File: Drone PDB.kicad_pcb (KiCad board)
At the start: 2 copper layers, 8 parts, among them CN1 XT60PW-M, CN2 XT60PW-M, CN3 XT60PW-M, CN4 XT60PW-M, CN5 XT60PW-M, CN6 XT60PW-M, CN7 XT60PW-M, CN8 XT60PW-M

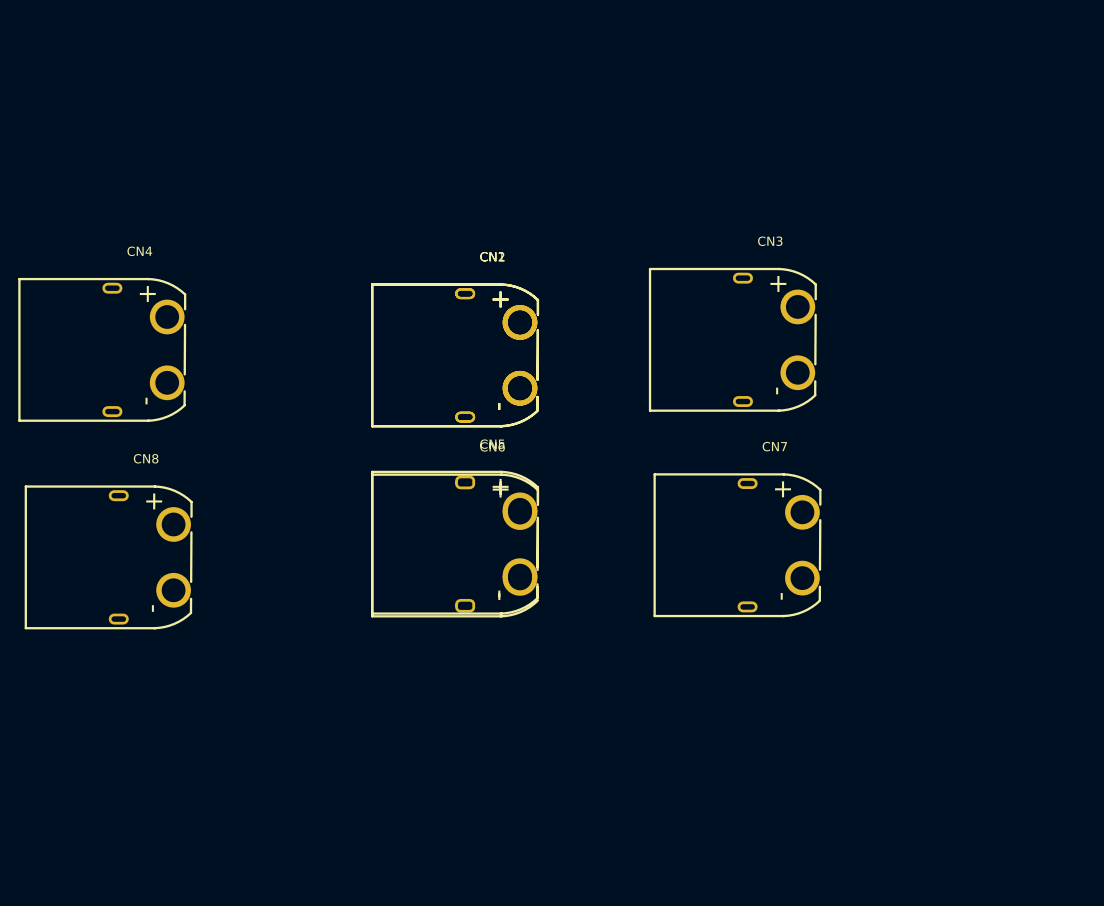
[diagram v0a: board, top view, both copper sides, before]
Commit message: drone pcb done
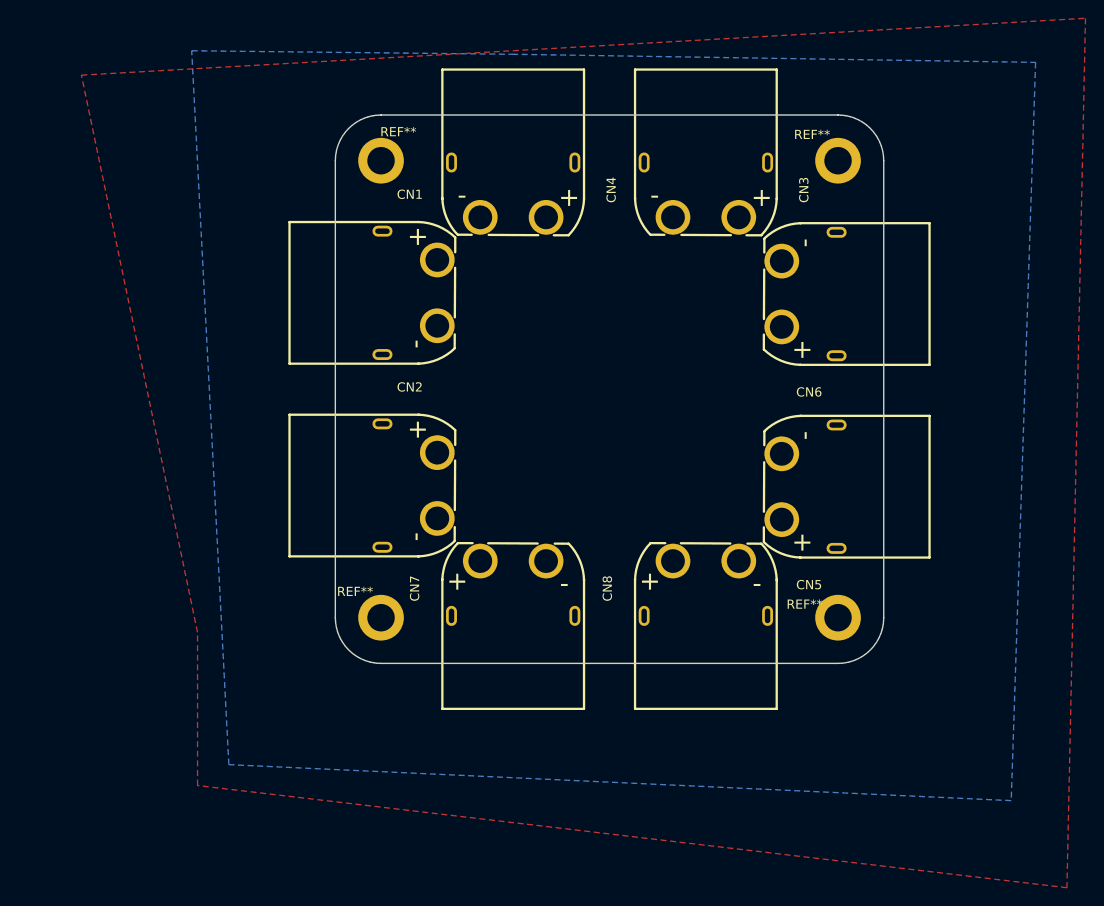
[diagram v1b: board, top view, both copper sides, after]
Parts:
- added REF**: 3mm HOLE, easyeda2kicad:3mm HOLE, F.Cu at (200.0, 50.0)
- added REF**: 3mm HOLE, easyeda2kicad:3mm HOLE, F.Cu at (150.0, 100.0)
- added REF**: 3mm HOLE, easyeda2kicad:3mm HOLE, F.Cu at (200.0, 100.0)
- added REF**: 3mm HOLE, easyeda2kicad:3mm HOLE, F.Cu at (150.0, 50.0)
- moved CN8 61.3 mm to (185.5, 96.8), turned to 90 degrees
- moved CN4 44.4 mm to (164.5, 53.2), turned to -90 degrees
- moved CN6 44.2 mm to (196.8, 64.6), turned to 180 degrees
- moved CN5 35.2 mm to (196.8, 85.7), turned to 180 degrees
- moved CN7 29.0 mm to (164.5, 96.8), turned to 90 degrees
- moved CN3 17.9 mm to (185.5, 53.2), turned to -90 degrees
- moved CN2 16.9 mm to (153.2, 85.5)
- moved CN1 11.3 mm to (153.2, 64.5)
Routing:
- added copper zone on B.Cu, net GND
- added copper zone on F.Cu, net VCC
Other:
- board outline added: 60 x 60 mm
